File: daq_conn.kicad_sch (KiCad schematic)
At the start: 65 parts

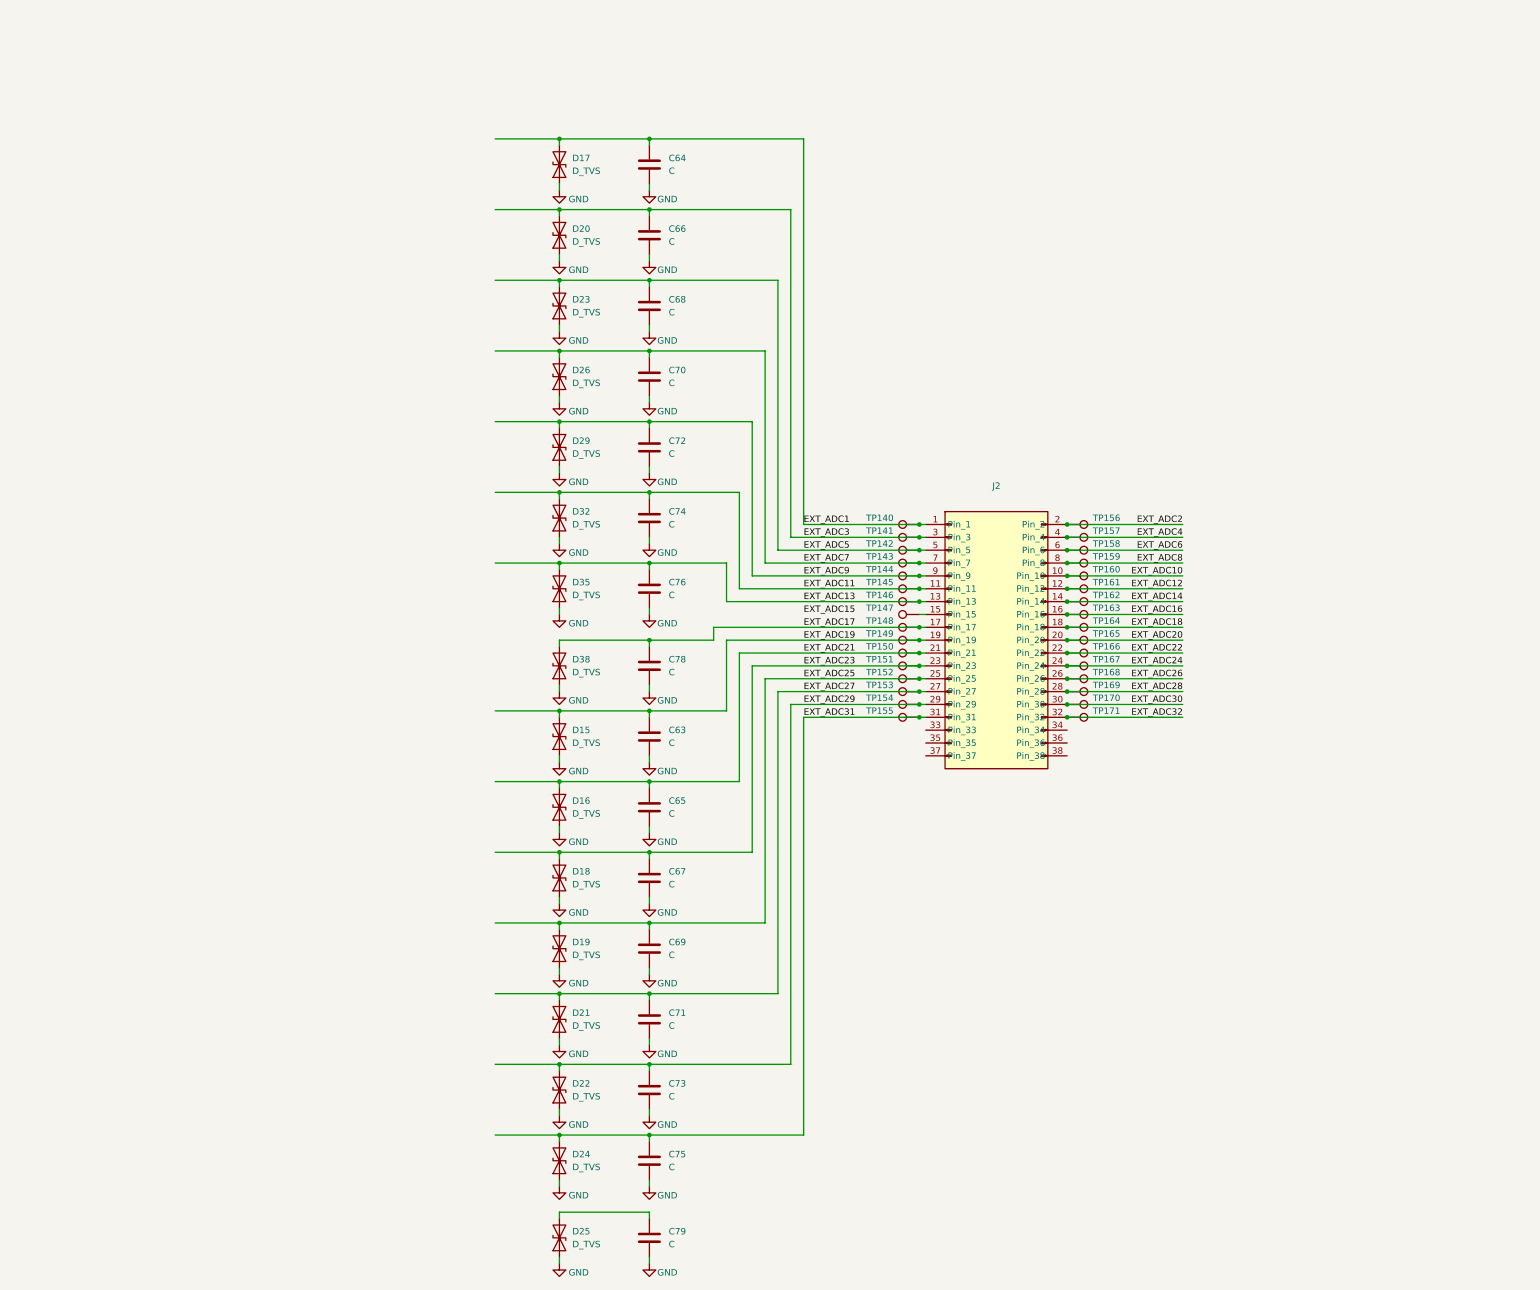
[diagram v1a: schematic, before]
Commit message: did stuff
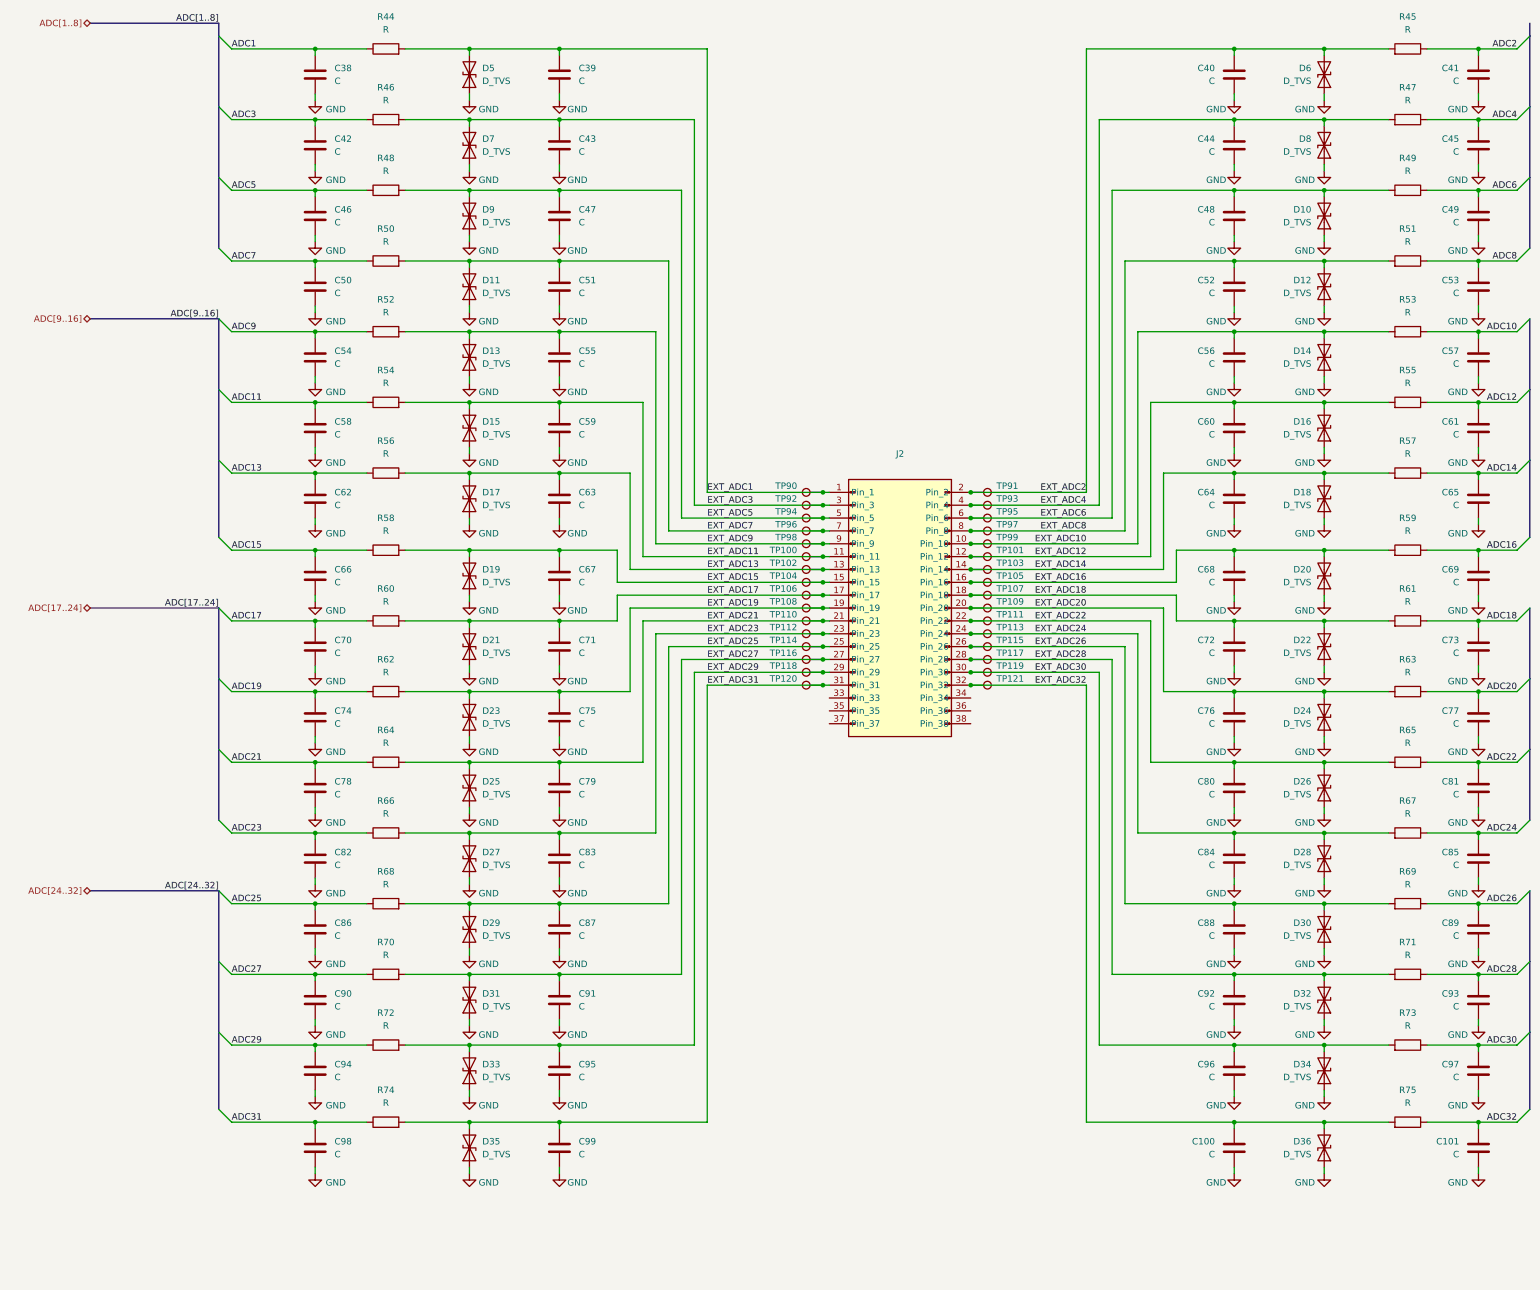
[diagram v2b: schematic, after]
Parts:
- added C100, C101, C38, C40, C41, C42, C44, C45, C46, C48, C49, C50, C52, C53, C54, C56, C57, C58, C60, C61, C62, C64, C65, C66, C68, C69, C70, C72, C73, C74, C76, C77, C78, C80, C81, C82, C84, C85, C86, C88, C89, C90, C92, C93, C94, C96, C97, C98: C, Capacitor_SMD:C_0402_1005Metric, symbol Device:C
- added D10, D12, D14, D16, D18, D20, D22, D24, D26, D28, D30, D32, D34, D36, D6, D8: D_TVS, Diode_SMD:D_SOD-923, symbol Device:D_TVS
- added R44, R45, R46, R47, R48, R49, R50, R51, R52, R53, R54, R55, R56, R57, R58, R59, R60, R61, R62, R63, R64, R65, R66, R67, R68, R69, R70, R71, R72, R73, R74, R75: R, Resistor_SMD:R_0603_1608Metric, symbol Device:R
- C39: renamed from C64; footprint (none) -> Capacitor_SMD:C_0402_1005Metric
- C43: renamed from C66; footprint (none) -> Capacitor_SMD:C_0402_1005Metric
- C47: renamed from C68; footprint (none) -> Capacitor_SMD:C_0402_1005Metric
- C51: renamed from C70; footprint (none) -> Capacitor_SMD:C_0402_1005Metric
- C55: renamed from C72; footprint (none) -> Capacitor_SMD:C_0402_1005Metric
- C59: renamed from C74; footprint (none) -> Capacitor_SMD:C_0402_1005Metric
- C63: renamed from C76; footprint (none) -> Capacitor_SMD:C_0402_1005Metric
- C67: renamed from C78; footprint (none) -> Capacitor_SMD:C_0402_1005Metric
- C71: renamed from C63; footprint (none) -> Capacitor_SMD:C_0402_1005Metric
- C75: renamed from C65; footprint (none) -> Capacitor_SMD:C_0402_1005Metric
- C79: renamed from C67; footprint (none) -> Capacitor_SMD:C_0402_1005Metric
- C83: renamed from C69; footprint (none) -> Capacitor_SMD:C_0402_1005Metric
- C87: renamed from C71; footprint (none) -> Capacitor_SMD:C_0402_1005Metric
- C91: renamed from C73; footprint (none) -> Capacitor_SMD:C_0402_1005Metric
- C95: renamed from C75; footprint (none) -> Capacitor_SMD:C_0402_1005Metric
- C99: renamed from C79; footprint (none) -> Capacitor_SMD:C_0402_1005Metric
- D11: renamed from D26; footprint (none) -> Diode_SMD:D_SOD-923
- D13: renamed from D29; footprint (none) -> Diode_SMD:D_SOD-923
- D15: renamed from D32; footprint (none) -> Diode_SMD:D_SOD-923
- D17: renamed from D35; footprint (none) -> Diode_SMD:D_SOD-923
- D19: renamed from D38; footprint (none) -> Diode_SMD:D_SOD-923
- D21: renamed from D15; footprint (none) -> Diode_SMD:D_SOD-923
- D23: renamed from D16; footprint (none) -> Diode_SMD:D_SOD-923
- D25: renamed from D18; footprint (none) -> Diode_SMD:D_SOD-923
- D27: renamed from D19; footprint (none) -> Diode_SMD:D_SOD-923
- D29: renamed from D21; footprint (none) -> Diode_SMD:D_SOD-923
- D31: renamed from D22; footprint (none) -> Diode_SMD:D_SOD-923
- D33: renamed from D24; footprint (none) -> Diode_SMD:D_SOD-923
- D35: renamed from D25; footprint (none) -> Diode_SMD:D_SOD-923
- D5: renamed from D17; footprint (none) -> Diode_SMD:D_SOD-923
- D7: renamed from D20; footprint (none) -> Diode_SMD:D_SOD-923
- D9: renamed from D23; footprint (none) -> Diode_SMD:D_SOD-923
- renumbered TP145 to TP100, TP161 to TP101, TP146 to TP102, TP162 to TP103, TP147 to TP104, TP163 to TP105, TP148 to TP106, TP164 to TP107, TP149 to TP108, TP165 to TP109, TP150 to TP110, TP166 to TP111, TP151 to TP112, TP167 to TP113, TP152 to TP114, TP168 to TP115, TP153 to TP116, TP169 to TP117, TP154 to TP118, TP170 to TP119, TP155 to TP120, TP171 to TP121, TP140 to TP90, TP156 to TP91, TP141 to TP92, TP157 to TP93, TP142 to TP94, TP158 to TP95, TP143 to TP96, TP159 to TP97, TP144 to TP98, TP160 to TP99
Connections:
- net EXT_ADC1: now also R44.2
- net EXT_ADC10: now also C56.1, D14.2 (A2), R53.2
- net EXT_ADC11: now also R54.2
- net EXT_ADC12: now also C60.1, D16.2 (A2), R55.2
- net EXT_ADC13: now also R56.2
- net EXT_ADC14: now also C64.1, D18.2 (A2), R57.2
- net EXT_ADC15: now also C67.1, D19.2 (A2), J2.15 (Pin_15), TP104.1, R58.2
- net EXT_ADC16: now also C68.1, D20.2 (A2), R59.2
- net EXT_ADC17: now also C71.1, D21.2 (A2), R60.2; no longer C67.1, D19.2 (A2)
- net EXT_ADC18: now also C72.1, D22.2 (A2), R61.2
- net EXT_ADC19: now also C75.1, D23.2 (A2), R62.2; no longer C71.1, D21.2 (A2)
- net EXT_ADC2: now also C40.1, D6.2 (A2), R45.2
- net EXT_ADC20: now also C76.1, D24.2 (A2), R63.2
- net EXT_ADC21: now also C79.1, D25.2 (A2), R64.2; no longer C75.1, D23.2 (A2)
- net EXT_ADC22: now also C80.1, D26.2 (A2), R65.2
- net EXT_ADC23: now also C83.1, D27.2 (A2), R66.2; no longer C79.1, D25.2 (A2)
- net EXT_ADC24: now also C84.1, D28.2 (A2), R67.2
- net EXT_ADC25: now also C87.1, D29.2 (A2), R68.2; no longer C83.1, D27.2 (A2)
- net EXT_ADC26: now also C88.1, D30.2 (A2), R69.2
- net EXT_ADC27: now also C91.1, D31.2 (A2), R70.2; no longer C87.1, D29.2 (A2)
- net EXT_ADC28: now also C92.1, D32.2 (A2), R71.2
- net EXT_ADC29: now also C95.1, D33.2 (A2), R72.2; no longer C91.1, D31.2 (A2)
- net EXT_ADC3: now also R46.2
- net EXT_ADC30: now also C96.1, D34.2 (A2), R73.2
- net EXT_ADC31: now also C99.1, D35.2 (A2), R74.2; no longer C95.1, D33.2 (A2)
- net EXT_ADC32: now also C100.1, D36.2 (A2), R75.2
- net EXT_ADC4: now also C44.1, D8.2 (A2), R47.2
- net EXT_ADC5: now also R48.2
- net EXT_ADC6: now also C48.1, D10.2 (A2), R49.2
- net EXT_ADC7: now also R50.2
- net EXT_ADC8: now also C52.1, D12.2 (A2), R51.2
- net EXT_ADC9: now also R52.2
- net GND: now also C100.2, C101.2, C38.2, C40.2, C41.2, C42.2, C44.2, C45.2, C46.2, C48.2, C49.2, C50.2, C52.2, C53.2, C54.2, C56.2, C57.2, C58.2, C60.2, C61.2, C62.2, C64.2, C65.2, C66.2, C68.2, C69.2, C70.2, C72.2, C73.2, C74.2, C76.2, C77.2, C78.2, C80.2, C81.2, C82.2, C84.2, C85.2, C86.2, C88.2, C89.2, C90.2, C92.2, C93.2, C94.2, C96.2, C97.2, C98.2, D10.1 (A1), D12.1 (A1), D14.1 (A1), D16.1 (A1), D18.1 (A1), D20.1 (A1), D22.1 (A1), D24.1 (A1), D26.1 (A1), D28.1 (A1), D30.1 (A1), D32.1 (A1), D34.1 (A1), D36.1 (A1), D6.1 (A1), D8.1 (A1)
- new net ADC1: C38.1, R44.1
- new net ADC10: C57.1, R53.1
- new net ADC11: C58.1, R54.1
- new net ADC12: C61.1, R55.1
- new net ADC13: C62.1, R56.1
- new net ADC14: C65.1, R57.1
- new net ADC15: C66.1, R58.1
- new net ADC16: C69.1, R59.1
- new net ADC17: C70.1, R60.1
- new net ADC18: C73.1, R61.1
- new net ADC19: C74.1, R62.1
- new net ADC2: C41.1, R45.1
- new net ADC20: C77.1, R63.1
- new net ADC21: C78.1, R64.1
- new net ADC22: C81.1, R65.1
- new net ADC23: C82.1, R66.1
- new net ADC24: C85.1, R67.1
- new net ADC25: C86.1, R68.1
- new net ADC26: C89.1, R69.1
- new net ADC27: C90.1, R70.1
- new net ADC28: C93.1, R71.1
- new net ADC29: C94.1, R72.1
- new net ADC3: C42.1, R46.1
- new net ADC30: C97.1, R73.1
- new net ADC31: C98.1, R74.1
- new net ADC32: C101.1, R75.1
- new net ADC4: C45.1, R47.1
- new net ADC5: C46.1, R48.1
- new net ADC6: C49.1, R49.1
- new net ADC7: C50.1, R50.1
- new net ADC8: C53.1, R51.1
- new net ADC9: C54.1, R52.1
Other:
- moved on the sheet: C39, C43, C47, C51, C55, C59, C63, C67, C71, C75, C79, C83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
